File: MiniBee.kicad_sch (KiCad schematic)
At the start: 41 parts, among them J1 USB, J2 I2C, J3 RGB, J4 SK6812, P1 TC2030-CTX-Tag-Connect, SW1 DFU, U1 USBLC4SC6, U2 STM32WB5MMG, U3 SY8201

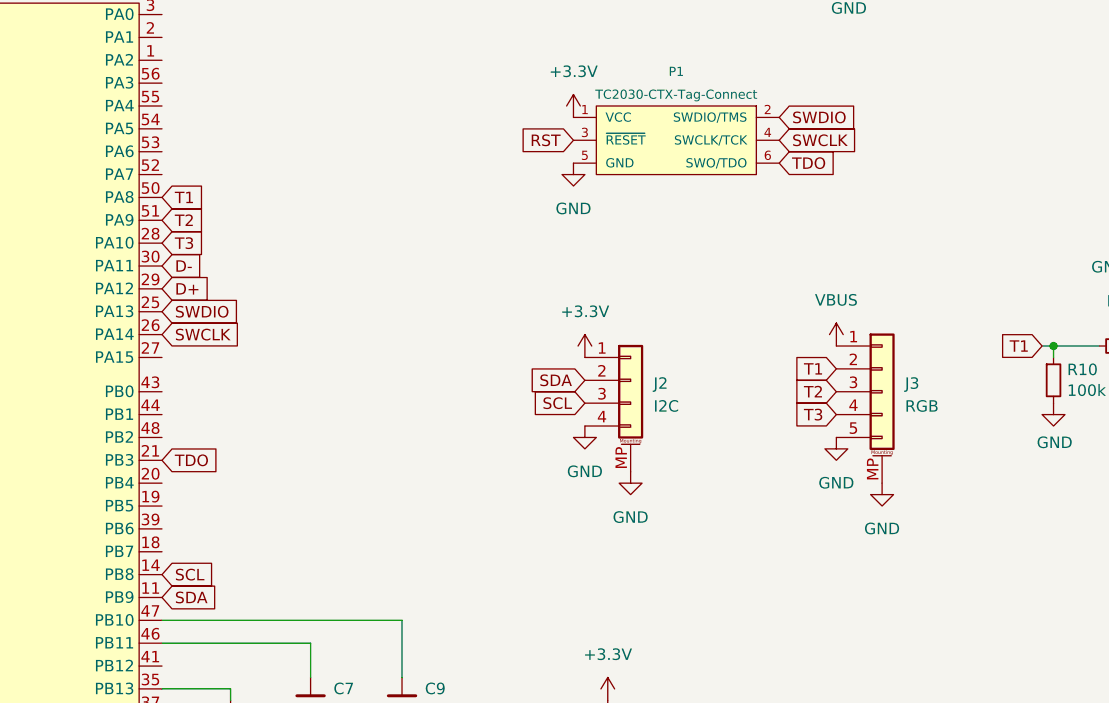
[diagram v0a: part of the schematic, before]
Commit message: updated project files
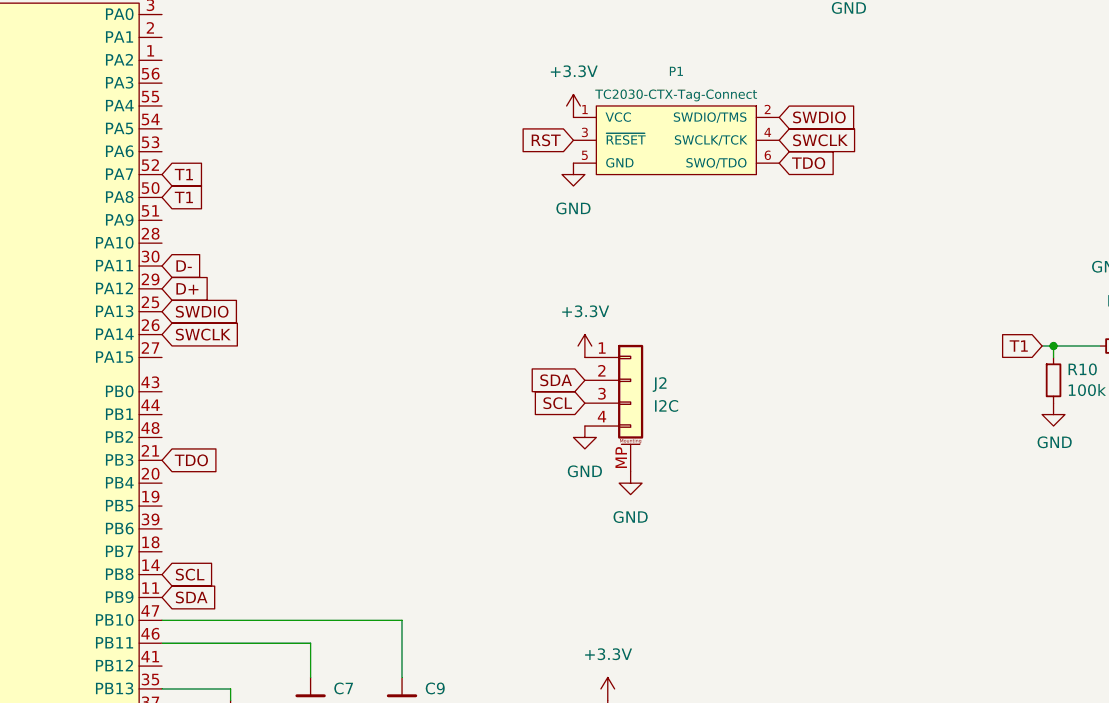
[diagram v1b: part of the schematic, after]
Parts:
- removed J3: RGB, Connector_Molex:Molex_PicoBlade_53398-0571_1x05-1MP_P1.25mm_Vertical, symbol Connector_Generic_MountingPin:Conn_01x05_MountingPin
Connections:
- net T1: now also U2.52 (PA7)
- net T2: no longer names the net of U2.51 (PA9)
- net T3: no longer names the net of U2.28 (PA10)
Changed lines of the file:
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@@
-    )
-  )
-  (global_label "T1" (shape input) (at 209.55 92.71 180) (fields_autoplaced)
-    (effects (font (size 1.27 1.27)) (justify right))
-    (property "Intersheet References" "${INTERSHEET_REFS}" (id 0) (at 204.9598 92.6306 0)
-      (effects (font (size 1.27 1.27)) (justify right) hide)
     )
   )
@@
     )
   )
-  (global_label "T3" (shape input) (at 209.55 97.79 180) (fields_autoplaced)
-    (effects (font (size 1.27 1.27)) (justify right))
-    (property "Intersheet References" "${INTERSHEET_REFS}" (id 0) (at 204.9598 97.7106 0)
-      (effects (font (size 1.27 1.27)) (justify right) hide)
-    )
-  )
   (global_label "D-" (shape input) (at 134.62 81.28 0) (fields_autoplaced)
     (effects (font (size 1.27 1.27)) (justify left))
@@
     )
   )
-  (global_label "T2" (shape input) (at 134.62 76.2 0) (fields_autoplaced)
-    (effects (font (size 1.27 1.27)) (justify left))
-    (property "Intersheet References" "${INTERSHEET_REFS}" (id 0) (at 139.2102 76.1206 0)
-      (effects (font (size 1.27 1.27)) (justify left) hide)
-    )
-  )
   (global_label "SCL" (shape input) (at 134.62 115.57 0) (fields_autoplaced)
     (effects (font (size 1.27 1.27)) (justify left))
@@
     )
   )
-  (global_label "T3" (shape input) (at 134.62 78.74 0) (fields_autoplaced)
-    (effects (font (size 1.27 1.27)) (justify left))
-    (property "Intersheet References" "${INTERSHEET_REFS}" (id 0) (at 139.2102 78.6606 0)
-      (effects (font (size 1.27 1.27)) (justify left) hide)
-    )
-  )
   (global_label "SDA" (shape input) (at 181.61 93.98 180) (fields_autoplaced)
     (effects (font (size 1.27 1.27)) (justify right))
@@
     )
   )
-  (global_label "T2" (shape input) (at 209.55 95.25 180) (fields_autoplaced)
-    (effects (font (size 1.27 1.27)) (justify right))
-    (property "Intersheet References" "${INTERSHEET_REFS}" (id 0) (at 204.9598 95.1706 0)
-      (effects (font (size 1.27 1.27)) (justify right) hide)
+  (global_label "T1" (shape input) (at 134.62 71.12 0) (fields_autoplaced)
+    (effects (font (size 1.27 1.27)) (justify left))
+    (property "Intersheet References" "${INTERSHEET_REFS}" (id 0) (at 139.2102 71.0406 0)
+      (effects (font (size 1.27 1.27)) (justify left) hide)
     )
   )
@@
     (pin "1")
   )
-  (symbol (lib_id "otter:GND") (at 214.63 105.41 0) (unit 1)
-    (in_bom yes) (on_board yes) (fields_autoplaced)
-    (property "Reference" "#PWR0134" (id 0) (at 214.63 111.76 0)
-      (effects (font (size 1.27 1.27)) hide)
-    )
-    (property "Value" "GND" (id 1) (at 214.63 110.49 0))
-    (property "Footprint" "" (id 2) (at 214.63 105.41 0)
-      (effects (font (size 1.524 1.524)))
-    )
-    (property "Datasheet" "" (id 3) (at 214.63 105.41 0)
-      (effects (font (size 1.524 1.524)))
-    )
-    (pin "1")
-  )
   (symbol (lib_id "LED:SK6812") (at 251.46 90.17 0) (unit 1)
     (in_bom yes) (on_board yes)
@@
     (pin "1")
     (pin "2")
-  )
-  (symbol (lib_id "power:VBUS") (at 209.55 90.17 0) (unit 1)
-    (in_bom yes) (on_board yes) (fields_autoplaced)
-    (property "Reference" "#PWR0135" (id 0) (at 209.55 93.98 0)
-      (effects (font (size 1.27 1.27)) hide)
-    )
-    (property "Value" "VBUS" (id 1) (at 209.55 85.09 0))
-    (property "Footprint" "" (id 2) (at 209.55 90.17 0)
-      (effects (font (size 1.27 1.27)) hide)
-    )
-    (property "Datasheet" "" (id 3) (at 209.55 90.17 0)
-      (effects (font (size 1.27 1.27)) hide)
-    )
-    (pin "1")
   )
   (symbol (lib_id "Device:C_Small") (at 265.43 33.02 180) (unit 1)
@@
     )
     (pin "1")
-  )
-  (symbol (lib_id "Connector_Generic_MountingPin:Conn_01x05_MountingPin") (at 214.63 95.25 0) (unit 1)
-    (in_bom yes) (on_board yes) (fields_autoplaced)
-    (property "Reference" "J3" (id 0) (at 217.17 94.3355 0)
-      (effects (font (size 1.27 1.27)) (justify left))
-    )
-    (property "Value" "RGB" (id 1) (at 217.17 96.8755 0)
-      (effects (font (size 1.27 1.27)) (justify left))
-    )
-    (property "Footprint" "Connector_Molex:Molex_PicoBlade_53398-0571_1x05-1MP_P1.25mm_Vertical" (id 2) (at 214.63 95.25 0)
-      (effects (font (size 1.27 1.27)) hide)
-    )
-    (property "Datasheet" "~" (id 3) (at 214.63 95.25 0)
-      (effects (font (size 1.27 1.27)) hide)
-    )
-    (pin "1")
-    (pin "2")
-    (pin "3")
-    (pin "4")
-    (pin "5")
-    (pin "MP")
   )
   (symbol (lib_id "Device:C_Small") (at 240.03 33.02 180) (unit 1)
@@
     (pin "1")
   )
-  (symbol (lib_id "otter:GND") (at 209.55 100.33 0) (unit 1)
-    (in_bom yes) (on_board yes) (fields_autoplaced)
-    (property "Reference" "#PWR0132" (id 0) (at 209.55 106.68 0)
-      (effects (font (size 1.27 1.27)) hide)
-    )
-    (property "Value" "GND" (id 1) (at 209.55 105.41 0))
-    (property "Footprint" "" (id 2) (at 209.55 100.33 0)
-      (effects (font (size 1.524 1.524)))
-    )
-    (property "Datasheet" "" (id 3) (at 209.55 100.33 0)
-      (effects (font (size 1.524 1.524)))
-    )
-    (pin "1")
-  )
   (symbol (lib_id "Device:R_Small") (at 196.85 33.02 0) (unit 1)
     (in_bom yes) (on_board yes)
@@
       (reference "#PWR0131") (unit 1) (value "+3.3V") (footprint "")
     )
-    (path "/eb541769-e0f7-4102-b851-fd5e1cea031a"
-      (reference "#PWR0132") (unit 1) (value "GND") (footprint "")
-    )
     (path "/ea20e0c6-9b5c-42b5-8ccd-0a7e05573f2a"
       (reference "#PWR0133") (unit 1) (value "GND") (footprint "")
     )
-    (path "/29a3ddb3-0c79-49d5-b650-4d8f4fff2161"
-      (reference "#PWR0134") (unit 1) (value "GND") (footprint "")
-    )
-    (path "/4efc5124-53b8-4b63-83b6-d24574f8d1be"
-      (reference "#PWR0135") (unit 1) (value "VBUS") (footprint "")
-    )
     (path "/8c11c305-2826-437a-b767-19837e2a3244"
       (reference "#PWR0136") (unit 1) (value "VBUS") (footprint "")
@@
       (reference "J2") (unit 1) (value "I2C") (footprint "Connector_Molex:Molex_PicoBlade_53398-0471_1x04-1MP_P1.25mm_Vertical")
     )
-    (path "/e2b20c39-9ad8-46e9-9e68-99fdf5a69024"
-      (reference "J3") (unit 1) (value "RGB") (footprint "Connector_Molex:Molex_PicoBlade_53398-0571_1x05-1MP_P1.25mm_Vertical")
-    )
     (path "/b64d4aa1-8926-47b1-953b-63be3e671648"
